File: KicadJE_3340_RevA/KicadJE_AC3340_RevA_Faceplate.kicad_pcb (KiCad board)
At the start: 2 copper layers, 40 x 128 mm, 20 parts

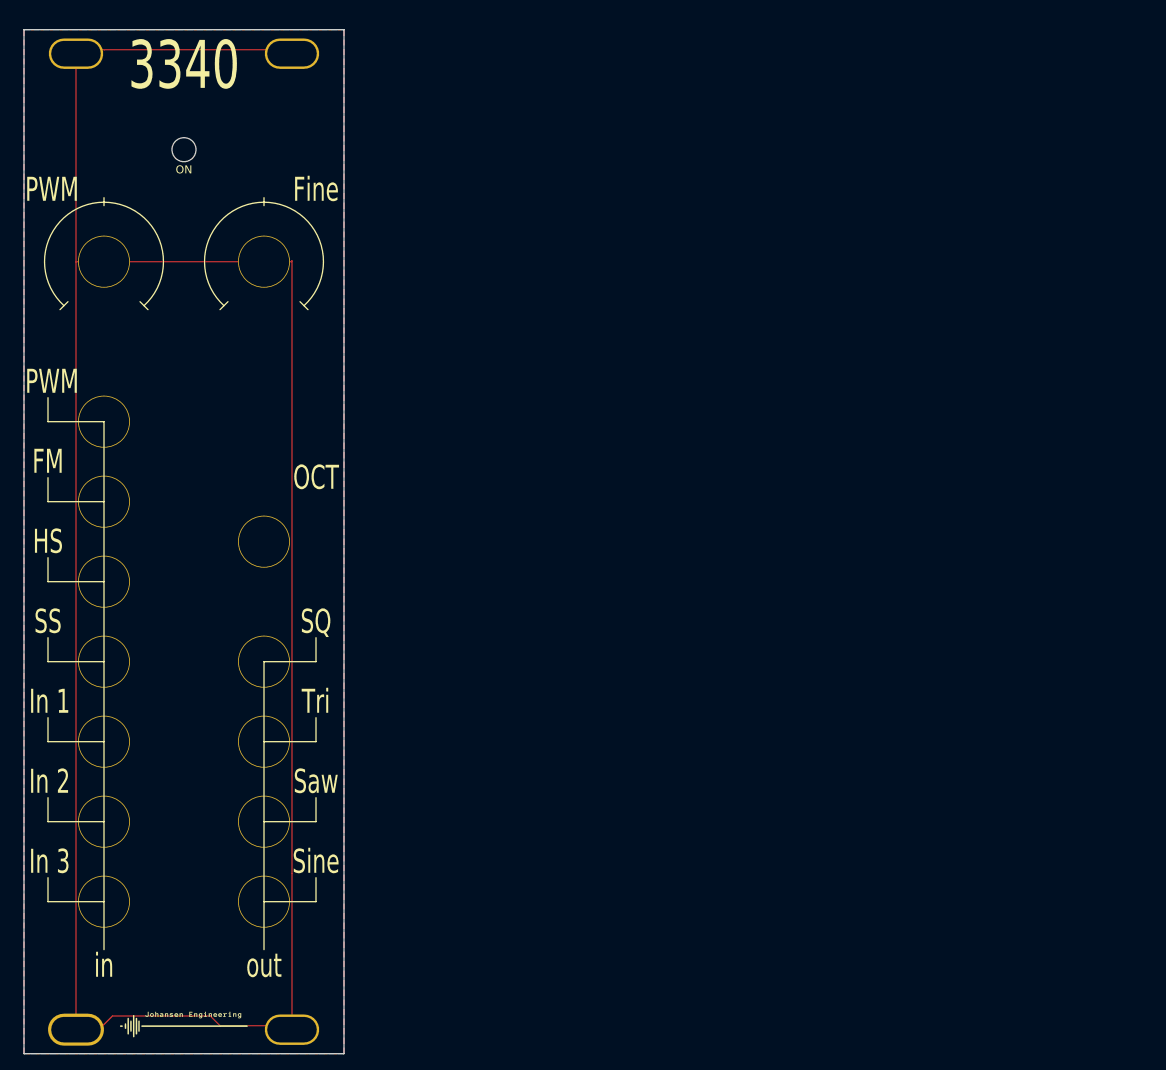
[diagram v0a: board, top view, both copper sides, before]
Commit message: JLC order number
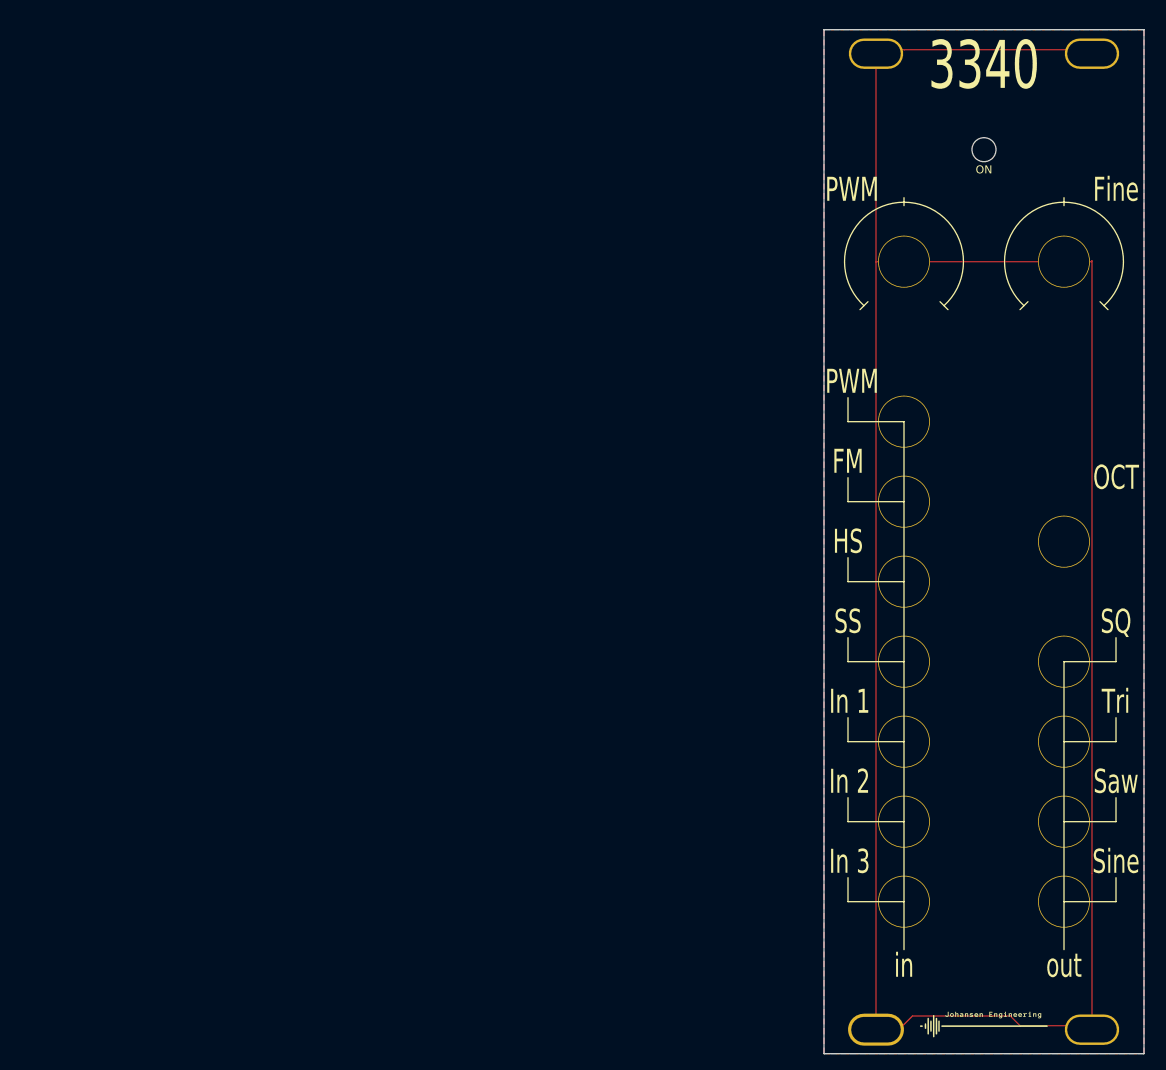
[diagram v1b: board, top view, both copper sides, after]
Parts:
- removed the REF** at (-40.0, 125.0)
- removed the REF** at (-40.0, 105.0)
- removed the REF** at (-40.0, 115.0)
- removed the REF** at (-20.0, 115.0)
- removed the REF** at (-20.0, 125.0)
- removed the REF** at (-20.0, 135.0)
- removed the REF** at (-40.0, 135.0)
- removed the REF** at (-40.0, 145.0)
- removed the REF** at (-20.0, 145.0)
- removed the REF** at (-16.5, 39.0)
- removed the REF** at (-43.5, 39.0)
- removed the REF** at (-16.5, 161.0)
- removed the REF** at (-20.0, 65.0)
- removed the REF** at (-40.0, 65.0)
- removed the REF** at (-40.0, 85.0)
- removed the REF** at (-40.0, 95.0)
- added REF**: 6,3mm inner, AJ:Jack_6m3, F.Cu at (60.0, 125.0)
- added REF**: 6,3mm inner, AJ:Jack_6m3, F.Cu at (60.0, 105.0)
- added REF**: 6,3mm inner, AJ:Jack_6m3, F.Cu at (60.0, 115.0)
- added REF**: 6,3mm inner, AJ:Jack_6m3, F.Cu at (80.0, 115.0)
- added REF**: 6,3mm inner, AJ:Jack_6m3, F.Cu at (80.0, 125.0)
- added REF**: 6,3mm inner, AJ:Jack_6m3, F.Cu at (80.0, 135.0)
- added REF**: 6,3mm inner, AJ:Jack_6m3, F.Cu at (60.0, 135.0)
- added REF**: 6,3mm inner, AJ:Jack_6m3, F.Cu at (60.0, 145.0)
- added REF**: 6,3mm inner, AJ:Jack_6m3, F.Cu at (80.0, 145.0)
- added REF**: MountingHole_Eurorack2, AJ:MountingHole_Eurorack2, F.Cu at (83.5, 39.0)
- added REF**: MountingHole_Eurorack2, AJ:MountingHole_Eurorack2, F.Cu at (56.5, 39.0)
- added REF**: MountingHole_Eurorack2, AJ:MountingHole_Eurorack2, F.Cu at (83.5, 161.0)
- added REF**: 6,3mm inner pot, AJ:Pot_6m3_scale1, F.Cu at (80.0, 65.0)
- added REF**: 6,3mm inner pot, AJ:Pot_6m3_scale1, F.Cu at (60.0, 65.0)
- added REF**: 6,3mm inner, AJ:Jack_6m3, F.Cu at (60.0, 85.0)
- added REF**: 6,3mm inner, AJ:Jack_6m3, F.Cu at (60.0, 95.0)
- moved G*** 100.0 mm to (70.0, 160.5)
- moved REF** 100.0 mm to (56.5, 161.0)
- moved REF** 100.0 mm to (80.0, 100.0)
- moved TP114 100.0 mm to (70.0, 51.0)
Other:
- board text added: "JLCJLCJLCJLC"
